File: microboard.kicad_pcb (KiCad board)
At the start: 2 copper layers, 95 parts, among them J10 Conn_01x01, J11 Conn_01x01, J12 Conn_01x10, J13 Conn_01x01, J14 Conn_01x12, J15 Conn_01x03, J17 Conn_01x01, J18 Conn_01x01, J2 Conn_01x10, J21 Conn_01x01_Socket, J22 Conn_01x01_Socket, J3 Conn_02x12, J39 Conn_01x10, J4 USB_C_Receptacle_USB2.0, J40 Conn_01x10, J41 Conn_01x10, J43 Conn_01x05, J44 Conn_01x09, J45 Conn_01x08, J5 Conn_01x04, J6 Conn_01x04, J7 Conn_01x05, J8 Conn_01x10, J9 Conn_01x01, SW1 SW_Push, SW2 SW_Push, SW7 RotaryEncoder_Switch, U1 USBLC6-2SC6, U2 ATSAMD21G18A-AUT, U3 LF33_TO220, U7 LF50_TO220, Y1 32768Hz

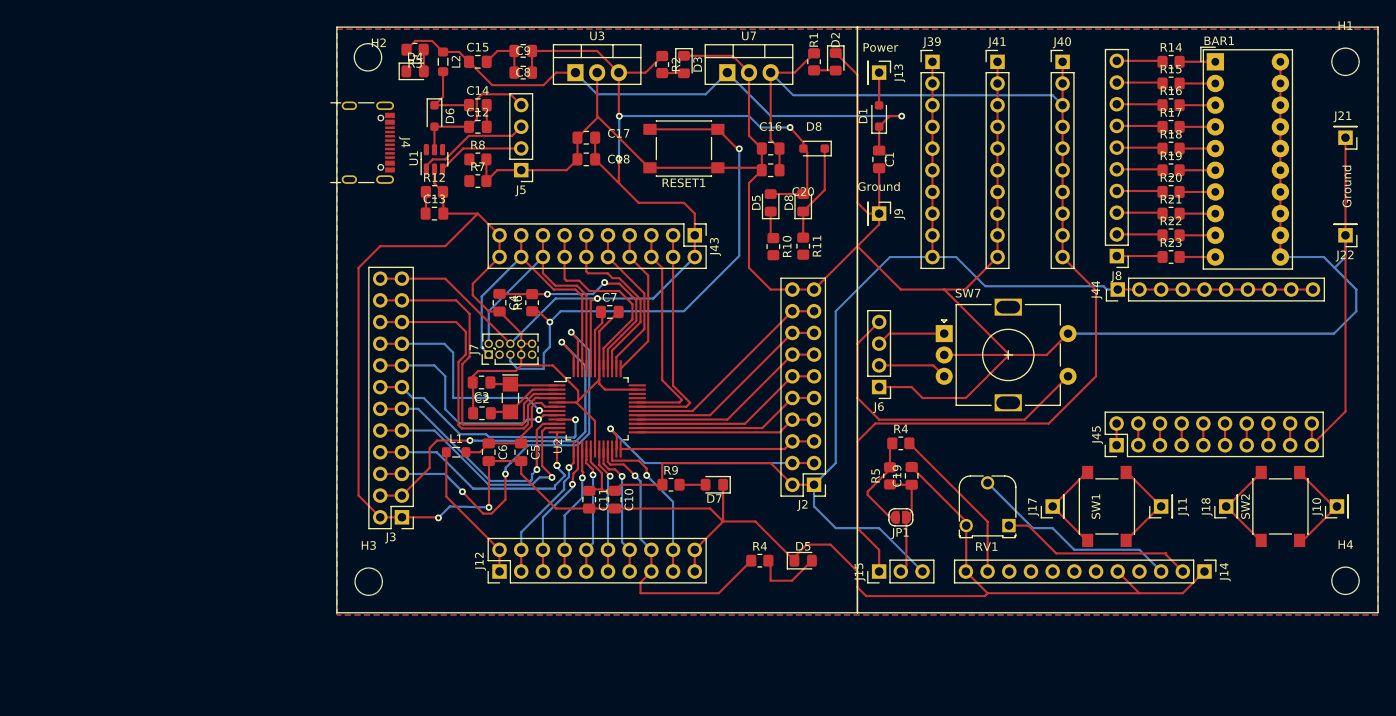
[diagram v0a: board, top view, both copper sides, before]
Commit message: almost final design
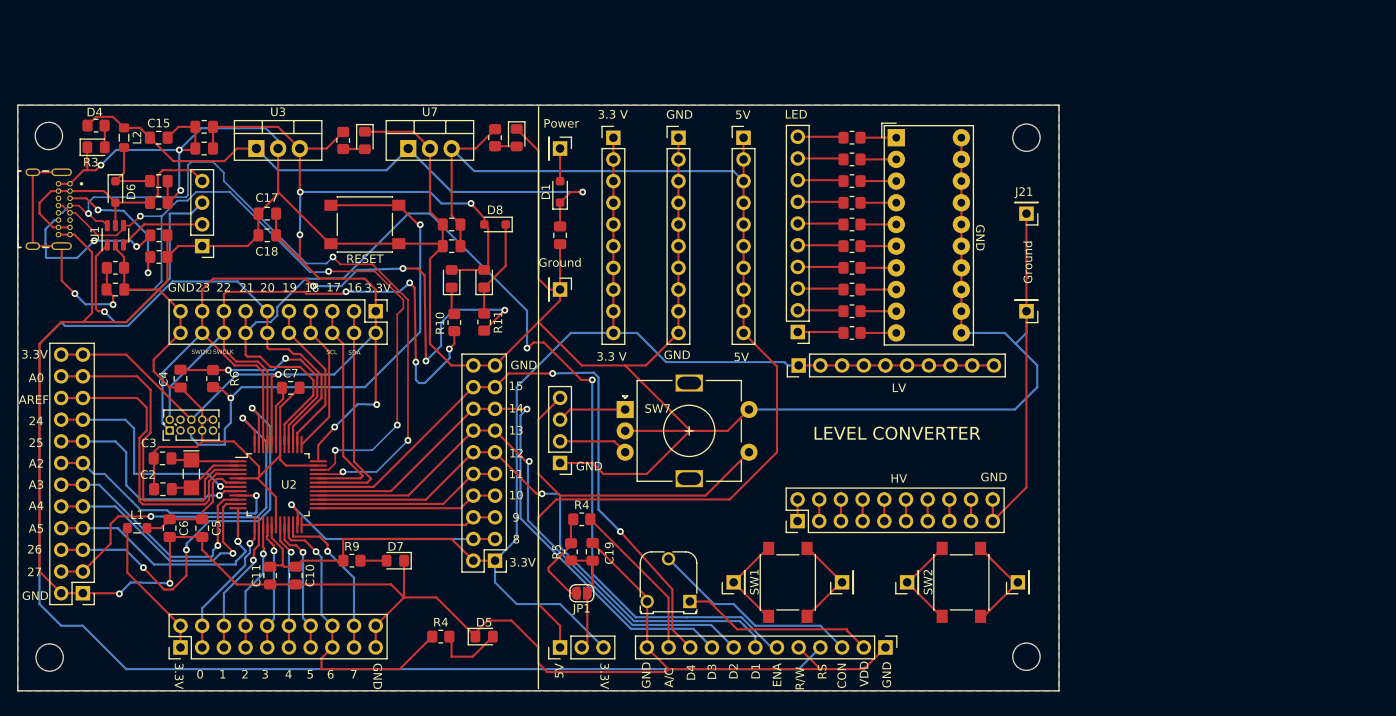
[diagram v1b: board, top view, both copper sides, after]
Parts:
- J4: value USB_C_Receptacle_USB2.0 -> USB4085-GF-A_REVB; footprint Connector_USB:USB_C_Receptacle_GCT_USB4105-xx-A_16P_TopMnt_Horizontal -> usb4085:GCT_USB4085-GF-A_REVB
- moved J4 38.9 mm to (91.4, 77.0)
- moved H2 38.5 mm to (93.3, 68.4)
- moved H4 38.4 mm to (207.8, 129.4)
- moved J12 38.4 mm to (108.7, 128.3)
- moved J15 38.4 mm to (153.1, 128.3)
- moved R15 38.4 mm to (187.3, 71.1)
- moved BAR1 38.4 mm to (192.5, 68.6)
- moved C1 38.4 mm to (153.1, 80.0)
- moved C11 38.4 mm to (119.2, 119.9)
- moved C13 38.4 mm to (101.1, 86.4)
- moved C16 38.4 mm to (140.4, 78.7)
- moved C17 38.4 mm to (118.8, 77.5)
- moved C18 38.4 mm to (118.8, 80.0)
- moved C19 38.4 mm to (156.9, 117.1)
- moved C20 38.4 mm to (140.4, 81.3)
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- renumbered RESET1 to RESET
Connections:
- C13 pad 1: Net-(J4-SHIELD) -> Net-(C13-Pad1)
- J14 pad 6: Pa28 -> PA28
- J2 pad 11: Net-(J2-Pin_11) -> PA18
- J2 pad 12: Net-(J2-Pin_11) -> PA18
- J2 pad 13: Net-(J2-Pin_13) -> PA19
- J2 pad 14: Net-(J2-Pin_13) -> PA19
- J2 pad 15: Net-(J2-Pin_15) -> PA20
- J2 pad 16: Net-(J2-Pin_15) -> PA20
- J2 pad 17: Net-(J2-Pin_17) -> PA21
- J2 pad 18: Net-(J2-Pin_17) -> PA21
- J4 pad A6: Net-(J5-Pin_2) -> D-
- J4 pad A7: Net-(J5-Pin_3) -> D+
- J4 pad B6: Net-(J5-Pin_2) -> D-
- J4 pad B7: Net-(J5-Pin_3) -> D+
- J4 pad S1: Net-(J4-SHIELD) -> Net-(C13-Pad1)
- J43 pad 11: Net-(J43-Pin_11) -> PA27
- J43 pad 12: Net-(J43-Pin_11) -> PA27
- J43 pad 13: Net-(J43-Pin_13) -> PA28
- J43 pad 14: Net-(J43-Pin_13) -> PA28
- J43 pad 15: Net-(J43-Pin_15) -> PA30
- J43 pad 16: Net-(J43-Pin_15) -> PA30
- J43 pad 17: Net-(J43-Pin_17) -> PA31
- J43 pad 18: Net-(J43-Pin_17) -> PA31
- J7 pad 1: Net-(J43-Pin_17) -> PA31
- J7 pad 2: Net-(J43-Pin_15) -> PA30
- R12 pad 1: Net-(J4-SHIELD) -> Net-(C13-Pad1)
- U2 pad 27: Net-(J2-Pin_11) -> PA18
- U2 pad 28: Net-(J2-Pin_13) -> PA19
- U2 pad 29: Net-(J2-Pin_15) -> PA20
- U2 pad 30: Net-(J2-Pin_17) -> PA21
- U2 pad 39: Net-(J43-Pin_11) -> PA27
- U2 pad 41: Net-(J43-Pin_13) -> PA28
- U2 pad 45: Net-(J43-Pin_15) -> PA30
- U2 pad 46: Net-(J43-Pin_17) -> PA31
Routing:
- net PA27: track 0.00 -> 179.1 mm
- net PA28: track 0.00 -> 129.6 mm, vias 0 -> 2
- net PA31: track 0.00 -> 91.8 mm, vias 0 -> 4
- net D+: track 0.00 -> 89.6 mm, vias 0 -> 4
- net D-: track 0.00 -> 86.4 mm, vias 0 -> 4
- net PA30: track 0.00 -> 77.6 mm, vias 0 -> 4
- net PA21: track 0.00 -> 74.6 mm, vias 0 -> 2
- net PA20: track 0.00 -> 70.2 mm, vias 0 -> 1
- net PA18: track 0.00 -> 67.4 mm, vias 0 -> 1
- net PA19: track 0.00 -> 66.5 mm, vias 0 -> 1
- net GND: track 613.9 -> 673.0 mm, vias 2 -> 5
- net Net-(J43-Pin_17): track 33.8 -> 0.00 mm
- net Net-(J43-Pin_15): track 32.0 -> 0.00 mm
- net Net-(C13-Pad1): track 0.00 -> 31.6 mm, vias 0 -> 2
- net Net-(J2-Pin_17): track 25.5 -> 0.00 mm
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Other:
- board outline added: 121.9 x 68.6 mm
- board text added: "0"
- board text added: "1"
- board text added: "10"
- board text added: "11"
- board text added: "12"
- board text added: "13"
- board text added: "14"
- board text added: "15"
- board text added: "16"
- board text added: "17"
- board text added: "18"
- board text added: "19"
- board text added: "2"
- board text added: "20"
- board text added: "21"
- board text added: "22"
- board text added: "23"
- board text added: "24"
- board text added: "25"
- board text added: "26"
- board text added: "27"
- board text added: "3"
- board text added: "3.3 V"
- board text added: "3.3V"
- board text added: "4"
- board text added: "5"
- board text added: "5V"
- board text added: "6"
- board text added: "7"
- board text added: "8"
- board text added: "9"
- board text added: "A/C"
- board text added: "A0"
- board text added: "A2"
- board text added: "A3"
- board text added: "A4"
- board text added: "A5"
- board text added: "AREF"
- board text added: "CON"
- board text added: "D1"
- board text added: "D2"
- board text added: "D3"
- board text added: "D4"
- board text added: "ENA"
- board text added: "GND"
- board text added: "HV"
- board text added: "LED"
- board text added: "LEVEL CONVERTER"
- board text added: "LV"
- board text added: "R/W"
- board text added: "RS"
- board text added: "SCL"
- board text added: "SDA"
- board text added: "SWCLK"
- board text added: "SWDIO"
- board text added: "VDD"
